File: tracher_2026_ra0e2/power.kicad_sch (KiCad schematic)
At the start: 46 parts, among them J3 Charger Connector, J4 Battery Connector, J5 UJC-H-G-SMT-2-P6-TR, Q1 MBT3946DW1T1, U3 MCP73831T-2ACI_OT

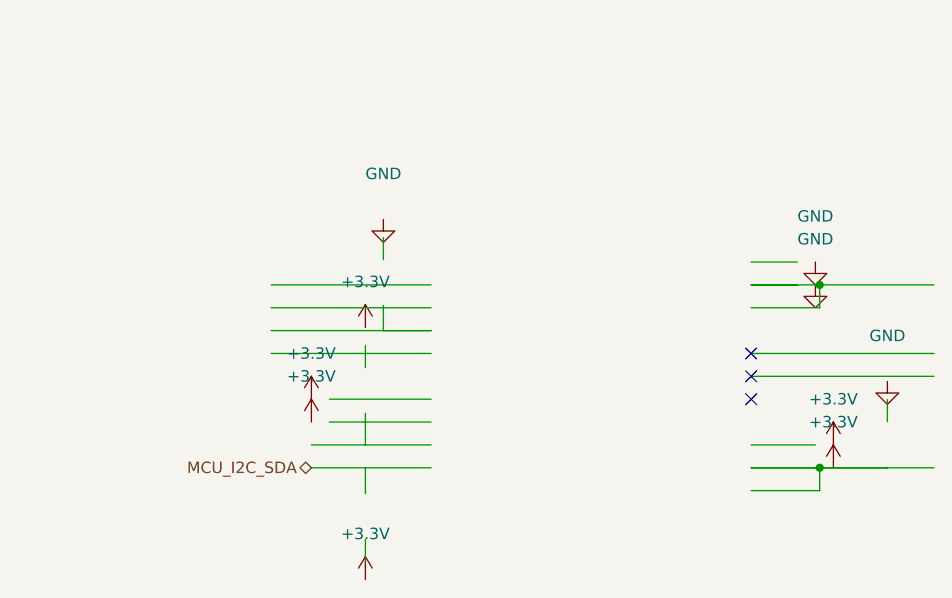
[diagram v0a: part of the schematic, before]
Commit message: removed Acc
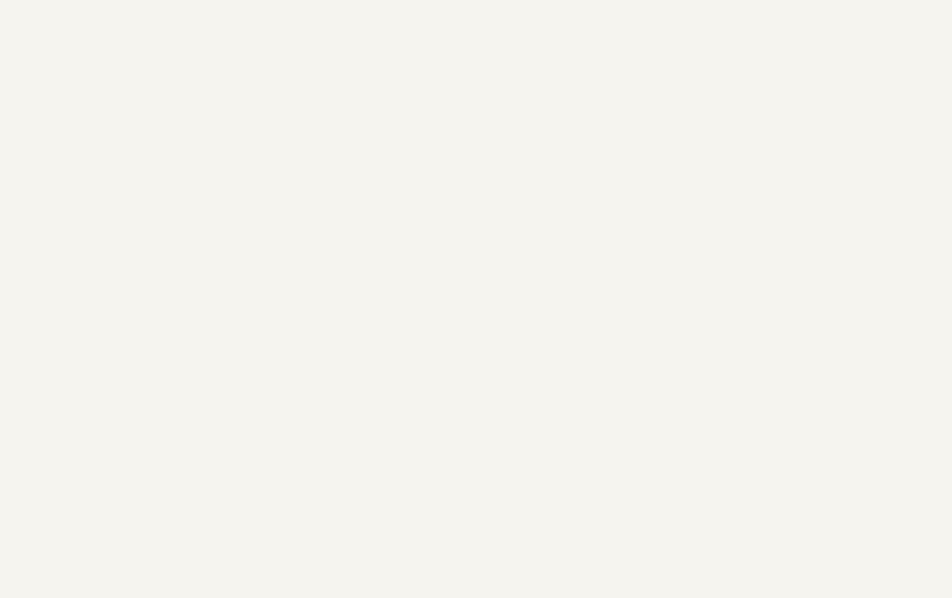
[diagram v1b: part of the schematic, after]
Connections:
- no-connect marks 3 -> 0
